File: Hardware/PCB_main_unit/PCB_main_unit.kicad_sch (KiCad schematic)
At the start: 49 parts, among them J1 Conn_01x03, J10 Conn_01x03, J11 Conn_01x03, J12 Conn_01x04, J13 Conn_01x07, J14 Conn_ST_STDC14, J15 Conn_01x03, J16 Conn_01x02, J2 Conn_01x03, J3 Conn_01x03, J4 Conn_01x03, J5 Conn_01x03, J6 Conn_01x03, J7 Conn_01x03, J8 Conn_01x03, J9 Conn_01x06, SW1 SW_SPDT, U2 STM32G474RETx, U3 AZ1117-3.3

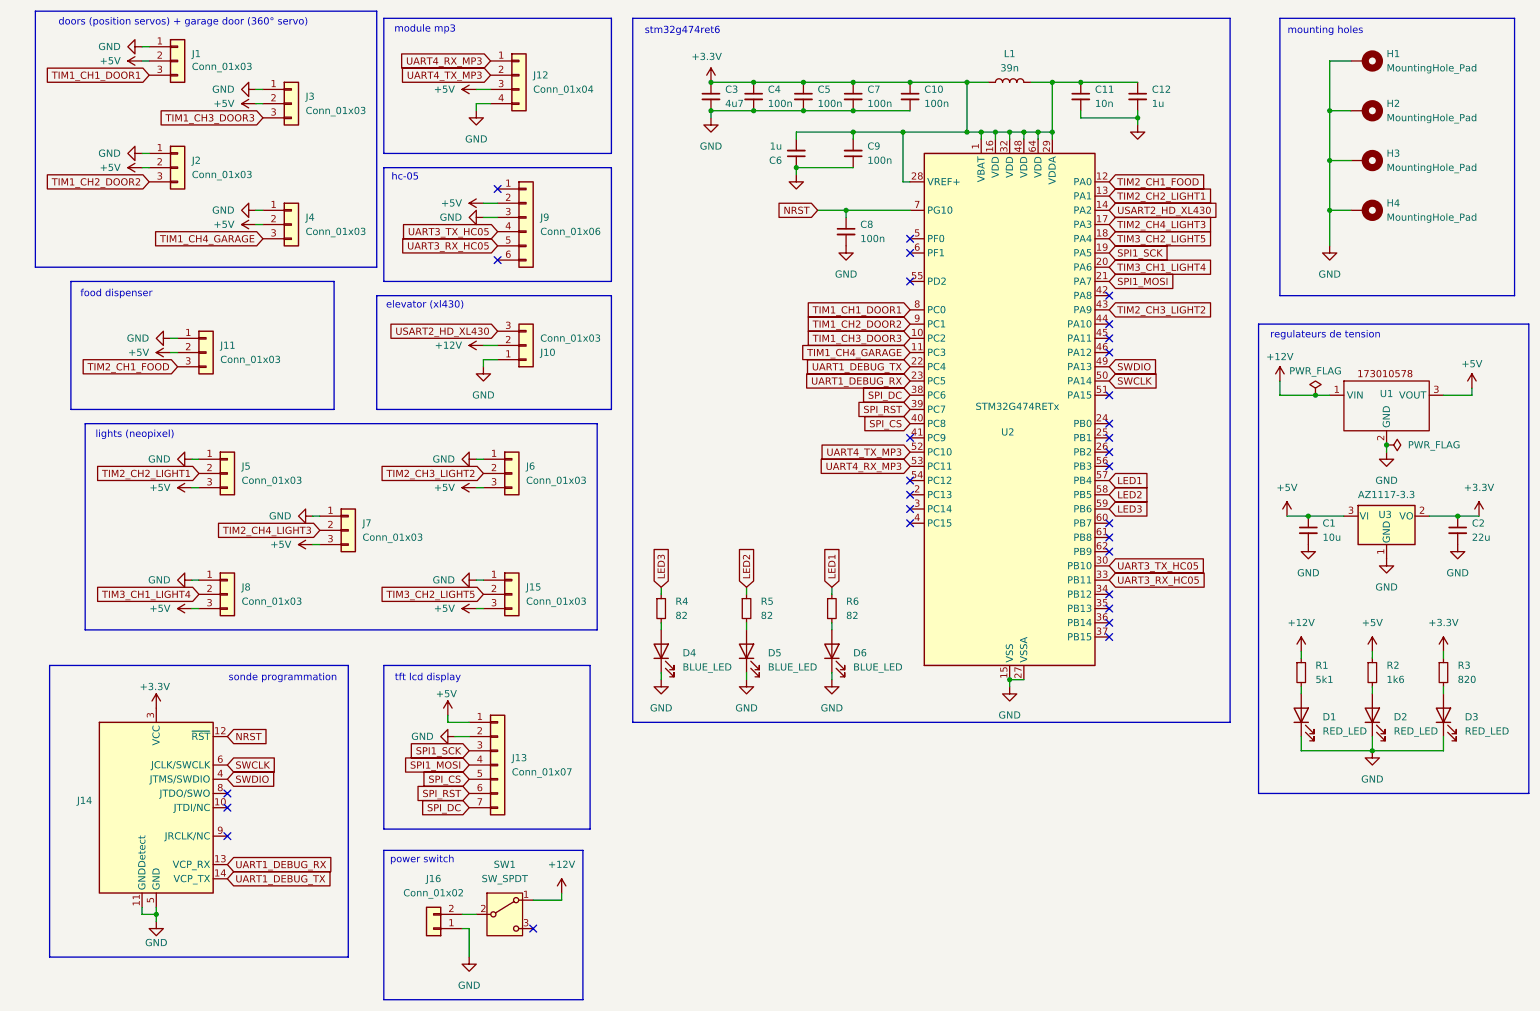
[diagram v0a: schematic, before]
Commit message: review sch
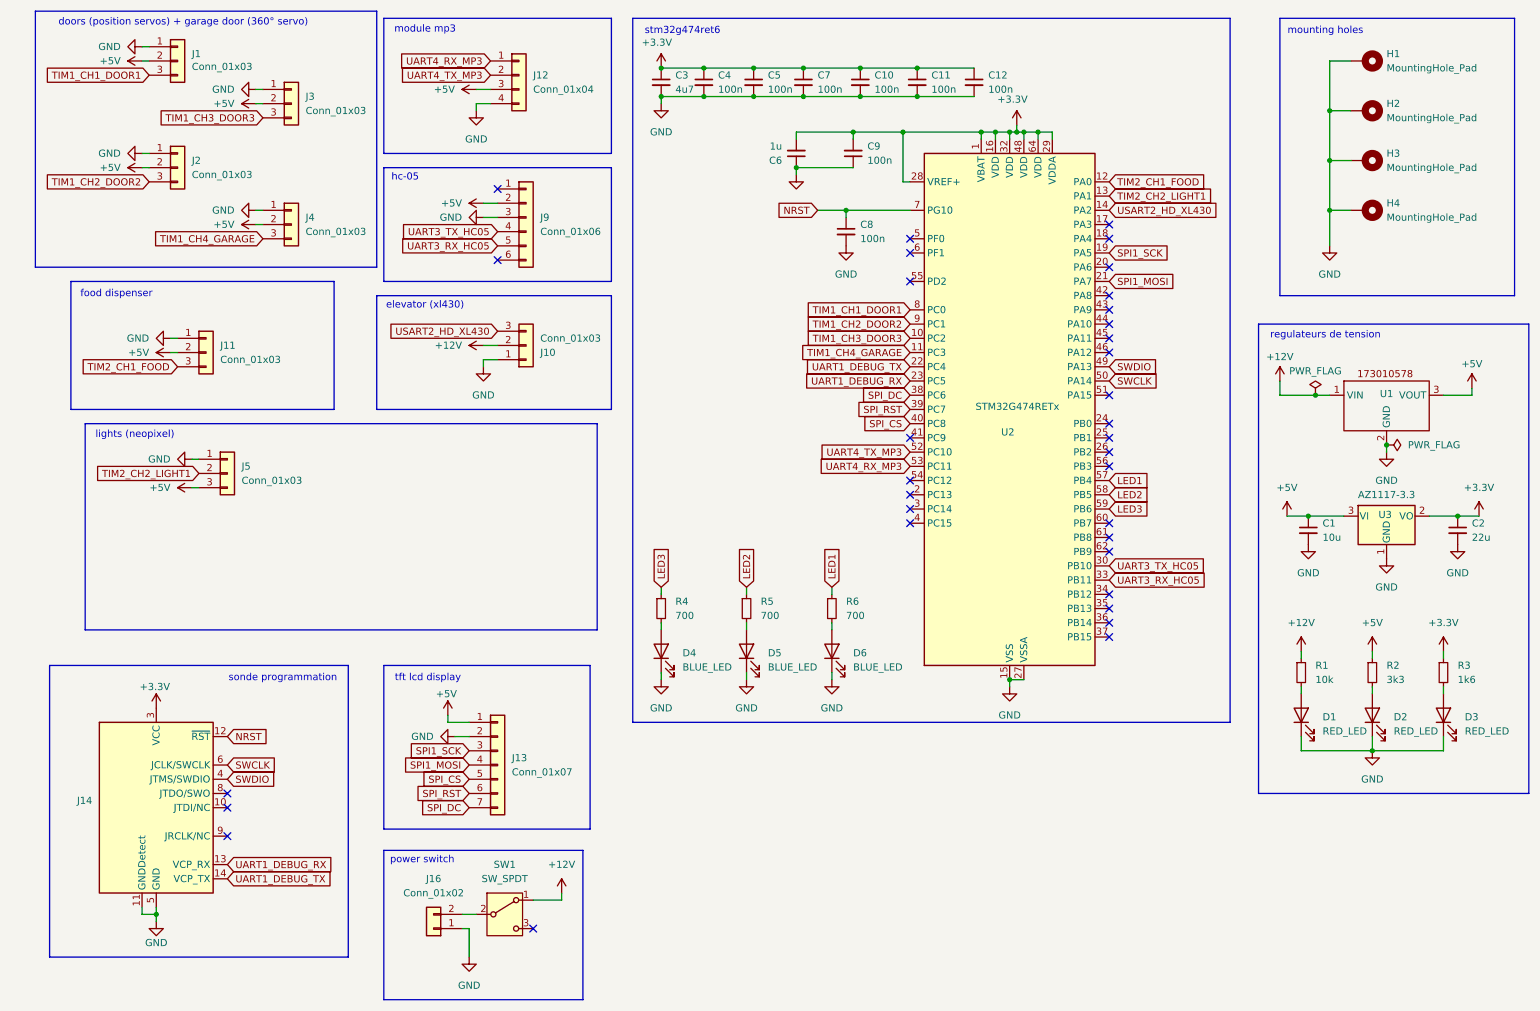
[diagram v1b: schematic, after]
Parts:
- removed J15, J6, J7, J8: Conn_01x03, Connector_JST:JST_EH_B3B-EH-A_1x03_P2.50mm_Vertical, symbol Connector_Generic:Conn_01x03
- removed L1: 39n, Inductor_SMD:L_0805_2012Metric, symbol Device:L
- C11: value 10n -> 100n
- C12: value 1u -> 100n; footprint Capacitor_SMD:C_0603_1608Metric -> Capacitor_SMD:C_0402_1005Metric_Pad0.74x0.62mm_HandSolder
- R1: value 5k1 -> 10k
- R2: value 1k6 -> 3k3
- R3: value 820 -> 1k6
- R4, R5, R6: value 82 -> 700
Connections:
- net TIM2_CH3_LIGHT2: no longer names the net of U2.43 (PA9)
- net TIM2_CH4_LIGHT3: no longer names the net of U2.17 (PA3)
- net TIM3_CH1_LIGHT4: no longer names the net of U2.20 (PA6)
- net TIM3_CH2_LIGHT5: no longer names the net of U2.18 (PA4)
- no-connect marks 30 -> 34
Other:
- moved on the sheet: C10, C3, C4, C5, C7

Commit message: applied changes
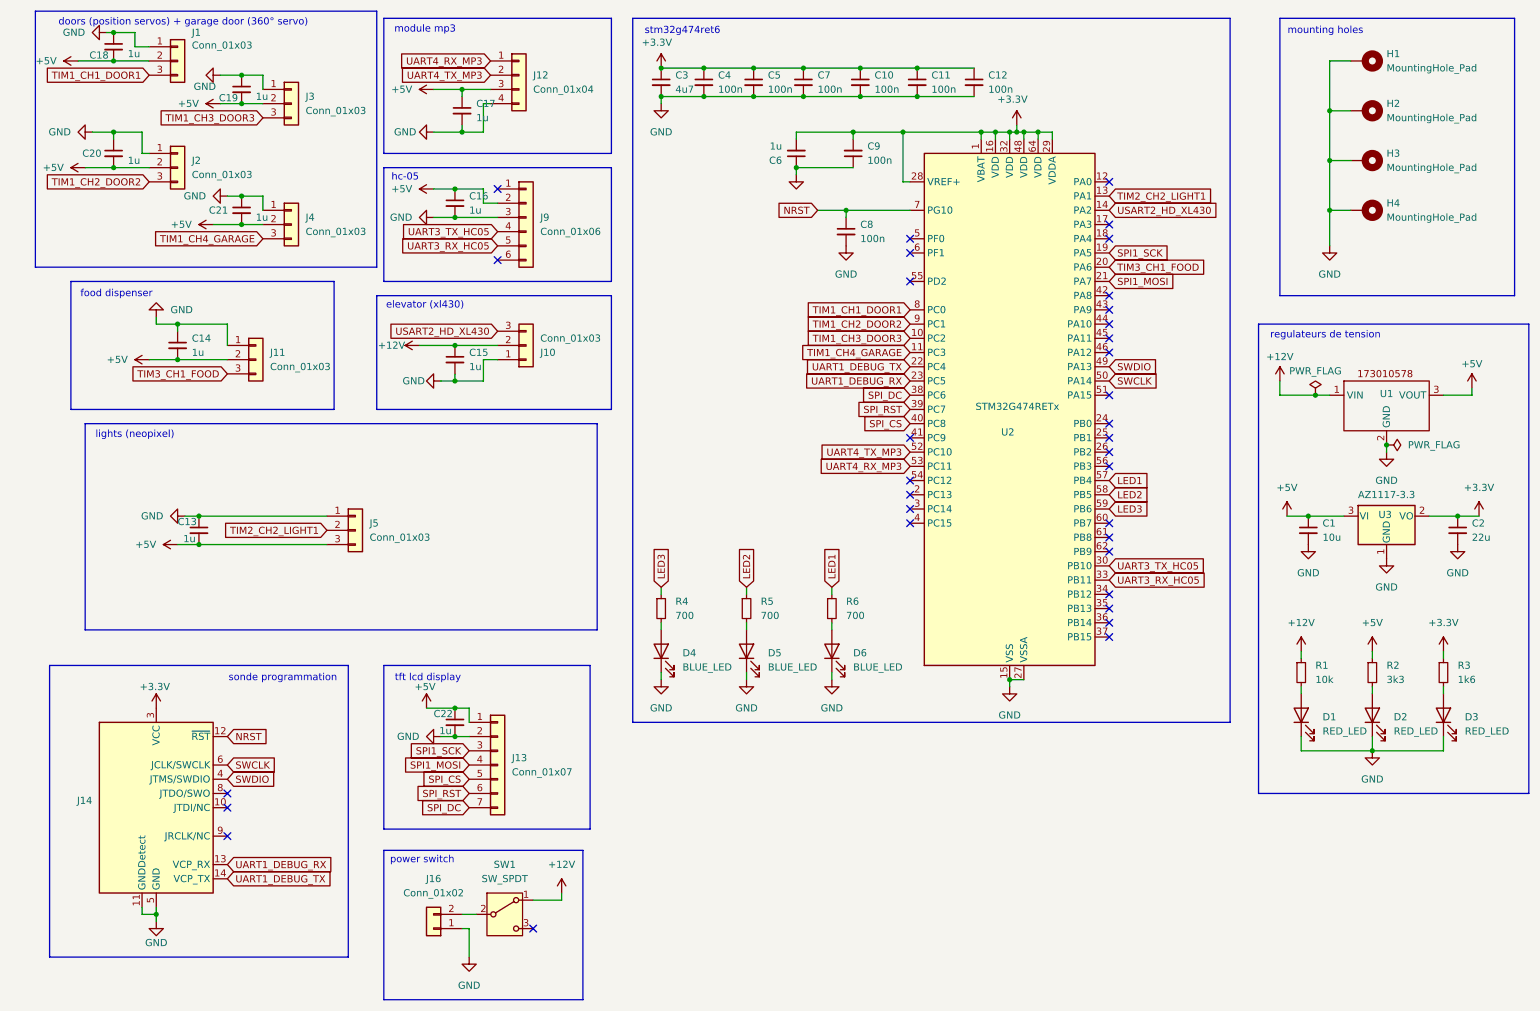
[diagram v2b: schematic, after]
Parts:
- added C13, C14, C15, C16, C17, C18, C19, C20, C21, C22: 1u, Capacitor_SMD:C_0603_1608Metric, symbol Device:C_Small
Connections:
- net +12V: now also C15.1
- net +5V: now also C13.2, C14.2, C16.1, C17.1, C18.2, C19.2, C20.2, C21.2, C22.1
- net GND: now also C13.1, C14.1, C15.2, C16.2, C17.2, C18.1, C19.1, C20.1, C21.1, C22.2
- net TIM3_CH1_FOOD: now reaches U2.20 (PA6)
- net TIM3_CH1_FOOD: now also J11.3 (Pin_3)
- net TIM2_CH1_FOOD: no longer names the net of U2.12 (PA0)
- net TIM2_CH1_FOOD: no longer J11.3 (Pin_3)
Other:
- moved on the sheet: J11, J5
